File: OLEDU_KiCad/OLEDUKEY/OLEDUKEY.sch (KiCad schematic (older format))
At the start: 19 parts, among them J1 USB_C_TYPE-C-31-M-12, SW91 SW_Push, SW92 SW_Push, SW93 Rotary_Encoder_Switch, SW94 Rotary_Encoder_Switch, U1 STM32F072RBTx, U2 2.42OLED, U3 AMS1117-3.3

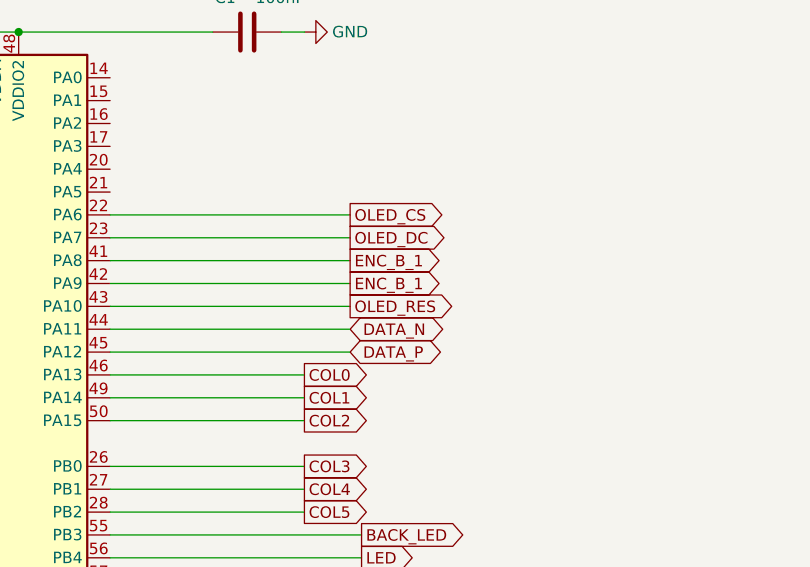
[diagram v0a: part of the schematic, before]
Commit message: production files added
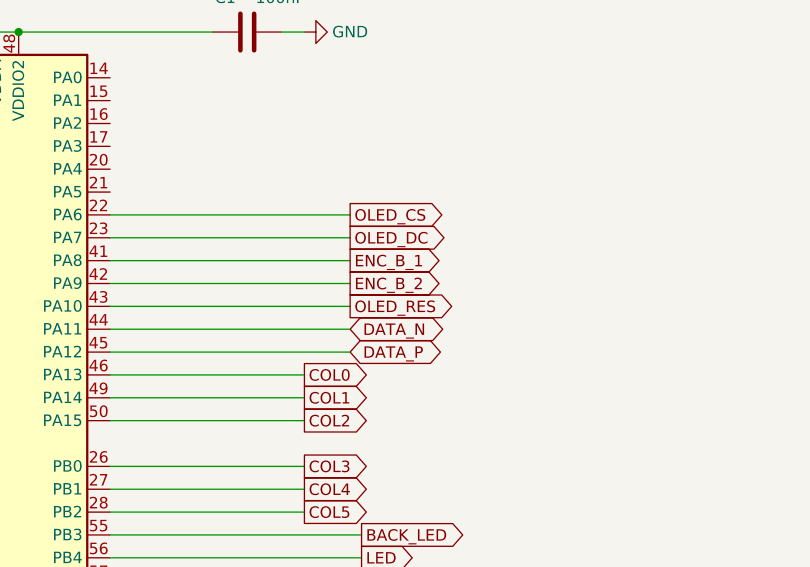
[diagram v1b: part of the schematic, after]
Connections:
- net ENC_B_1: no longer U1.42 (PA9)
- net ENC_B_2: now also U1.42 (PA9)
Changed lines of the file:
@@
 	3650 7850 4400 7850
 Text GLabel 6850 6450 2    50   Output ~ 0
-ENC_B_1
+ENC_B_2
 Wire Wire Line
 	5800 6450 6850 6450
